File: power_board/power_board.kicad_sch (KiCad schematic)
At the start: 0 parts

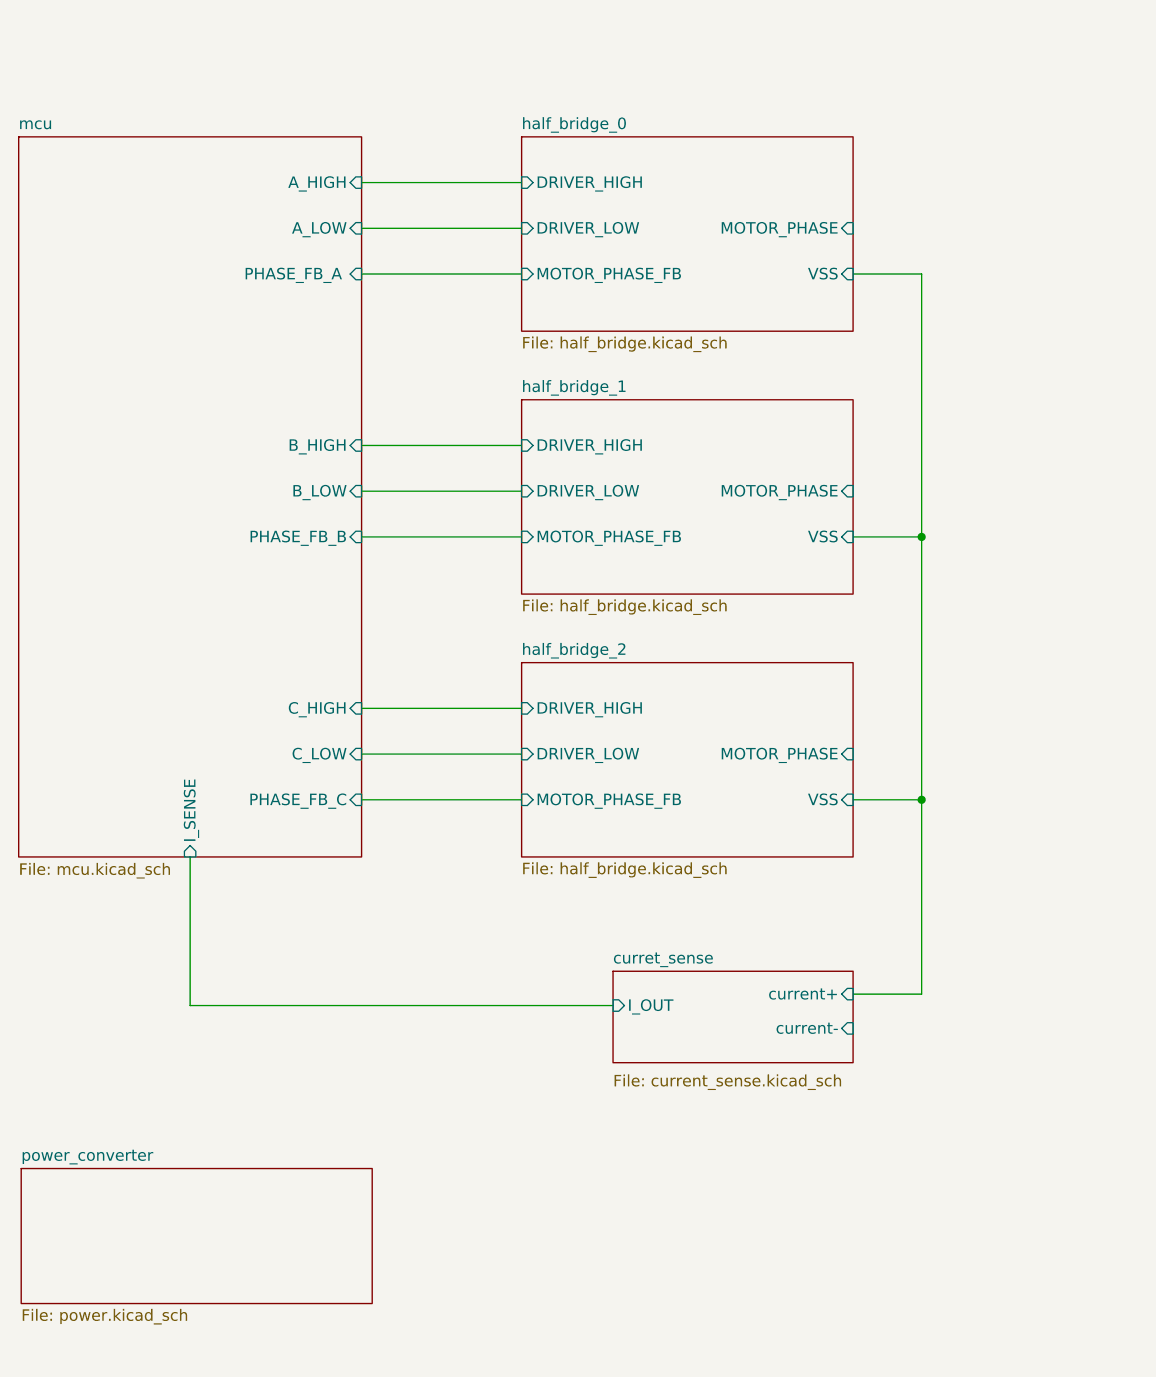
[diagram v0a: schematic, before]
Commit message: Complete sch design without check
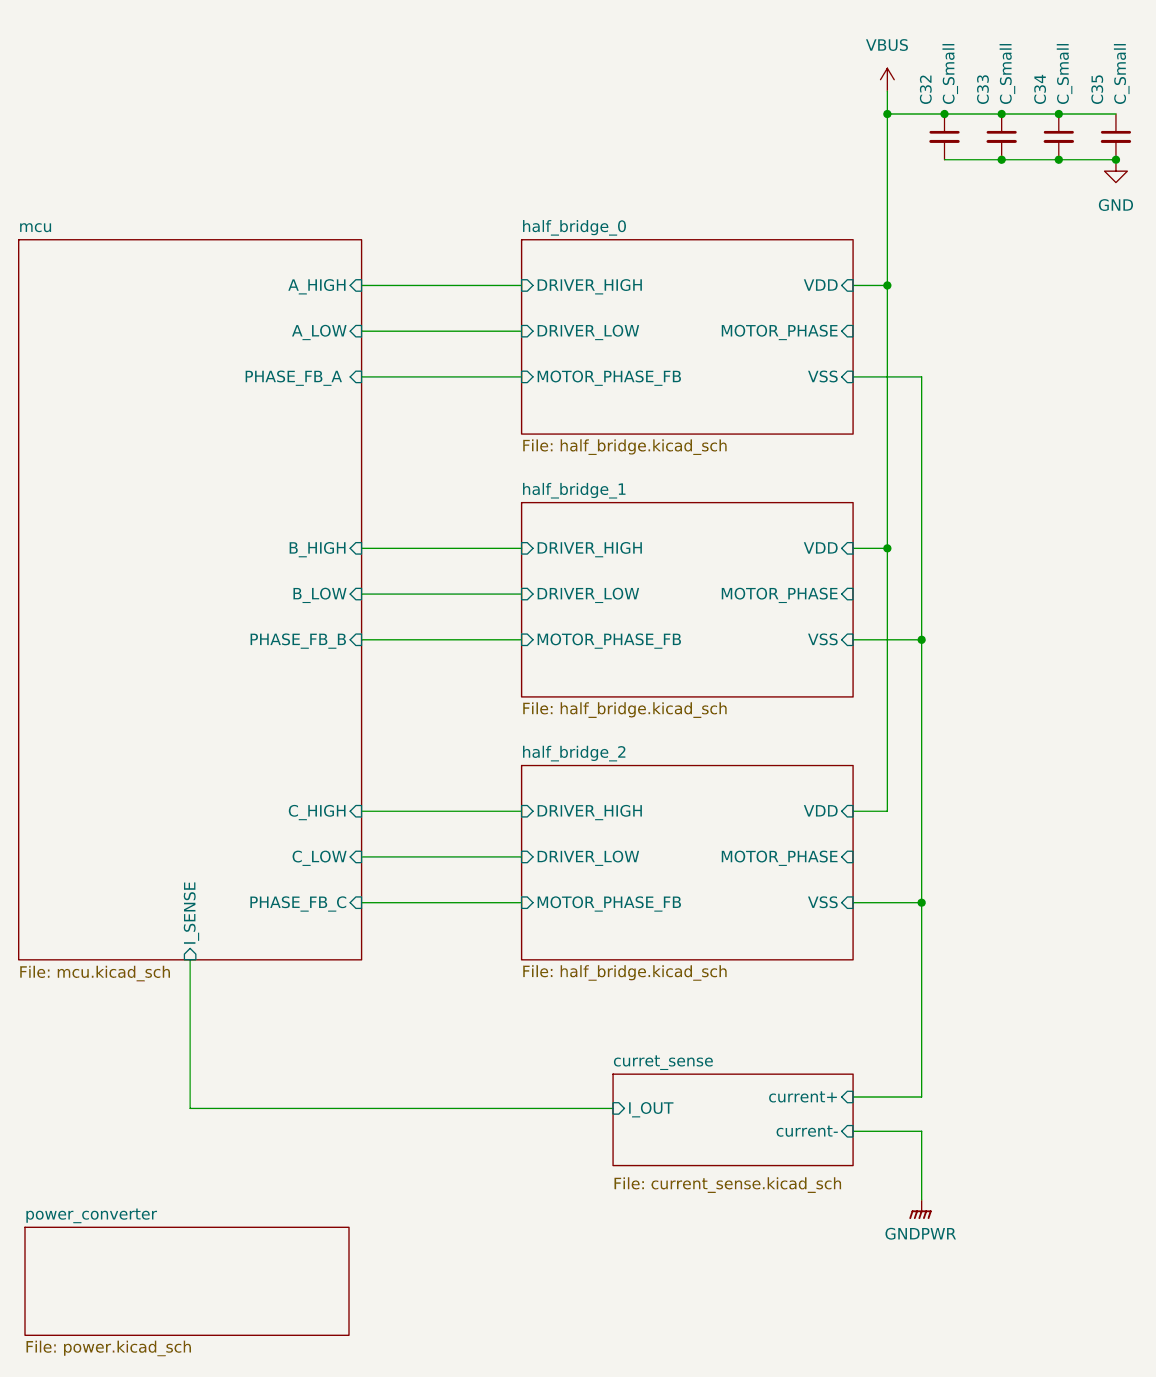
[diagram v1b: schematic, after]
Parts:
- added C32, C33, C34, C35: C_Small, Capacitor_SMD:C_2220_5750Metric, symbol Device:C_Small
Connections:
- new net GND: C32.2, C33.2, C34.2, C35.2
- new net VBUS: C32.1, C33.1, C34.1, C35.1
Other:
- sheet half_bridge_0 ports: added VDD; removed none
- sheet half_bridge_1 ports: added VDD; removed none
- sheet half_bridge_2 ports: added VDD; removed none
